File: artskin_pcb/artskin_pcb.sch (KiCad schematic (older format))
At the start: 3 parts

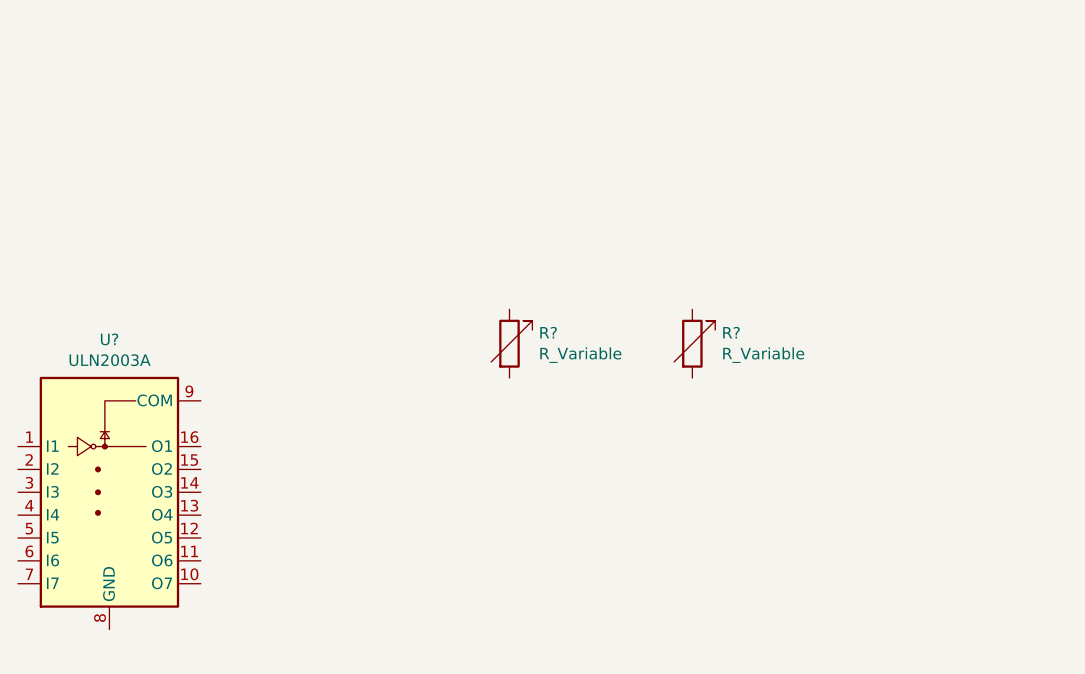
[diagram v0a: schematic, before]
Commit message: pcb: prototype design
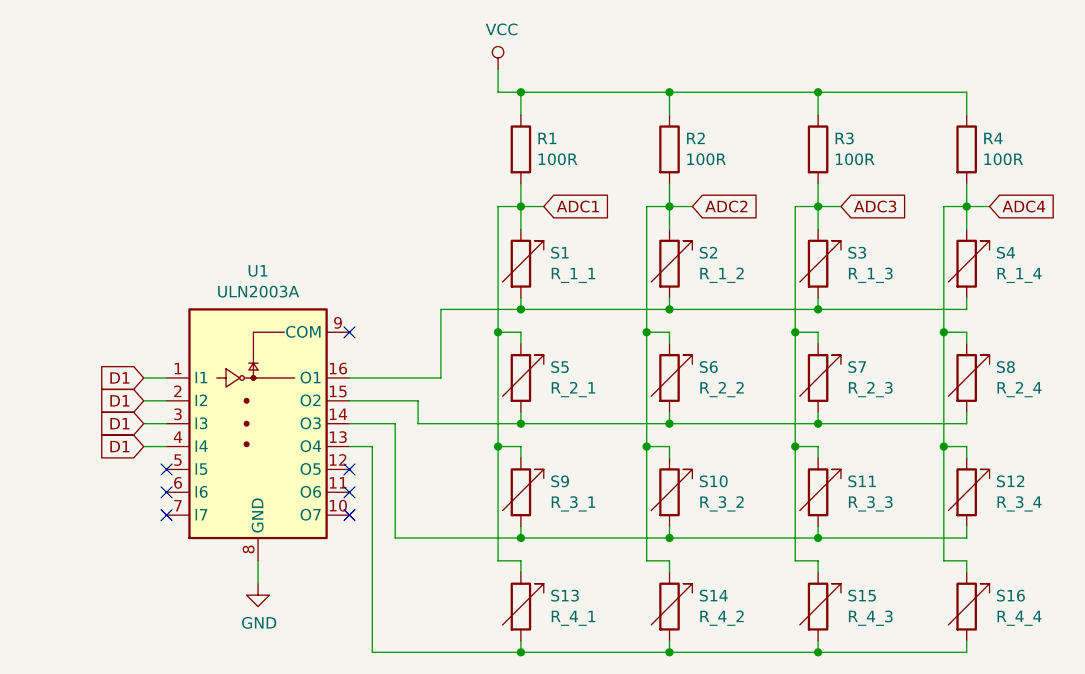
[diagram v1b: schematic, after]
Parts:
- removed R? (x2): R_Variable, symbol Device:R_Variable
- added R1, R2, R3, R4: 100R, symbol Device:R
- added S1: R_1_1, symbol Device:R_Variable
- added S10: R_3_2, symbol Device:R_Variable
- added S11: R_3_3, symbol Device:R_Variable
- added S12: R_3_4, symbol Device:R_Variable
- added S13: R_4_1, symbol Device:R_Variable
- added S14: R_4_2, symbol Device:R_Variable
- added S15: R_4_3, symbol Device:R_Variable
- added S16: R_4_4, symbol Device:R_Variable
- added S2: R_1_2, symbol Device:R_Variable
- added S3: R_1_3, symbol Device:R_Variable
- added S4: R_1_4, symbol Device:R_Variable
- added S5: R_2_1, symbol Device:R_Variable
- added S6: R_2_2, symbol Device:R_Variable
- added S7: R_2_3, symbol Device:R_Variable
- added S8: R_2_4, symbol Device:R_Variable
- added S9: R_3_1, symbol Device:R_Variable
- gave numbers to parts that had none: 1
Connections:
- net D1: now reaches U1.1 (I1)
- net D1: now also U1.2 (I2), U1.3 (I3), U1.4 (I4)
- net at U1.13 (O4): now also S13.2, S14.2, S15.2, S16.2
- net at U1.14 (O3): now also S10.2, S11.2, S12.2, S9.2
- net at U1.15 (O2): now also S5.2, S6.2, S7.2, S8.2
- net at U1.16 (O1): now also S1.2, S2.2, S3.2, S4.2
- net GND: now reaches U1.8 (GND)
- new net ADC1: R1.2, S1.1, S13.1, S5.1, S9.1
- new net ADC2: R2.2, S10.1, S14.1, S2.1, S6.1
- new net ADC3: R3.2, S11.1, S15.1, S3.1, S7.1
- new net ADC4: R4.2, S12.1, S16.1, S4.1, S8.1
- new net VCC: R1.1, R2.1, R3.1, R4.1
- no-connect marks 0 -> 7
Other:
- moved on the sheet: U1
